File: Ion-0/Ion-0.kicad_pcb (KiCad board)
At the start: 4 copper layers, 99 parts, among them J1 Beaglebone-green-P9, J10 Conn_Heater, J11 Conn_01x02, J12 Conn_01x02, J13 Conn_01x04, J2 Beaglebone-green-P8, J3 Conn_02x06_Odd_Even, J4 Conn_02x06_Odd_Even, J5 Conn_02x06_Odd_Even, J6 Coaxial_Small, J7 Conn_01x02, J8 Conn_Heater, J9 Conn_Heater, Q1 IRLML6244, Q2 IRLML6244, Q3 IRLML6244, Q4 IRLML6244, U2 LMT84DCK, U3 BNO085, U4 TCA9617ADGKR, U5 LMT84DCK, U6 MAX-M10M-00B, U7 TPS3850H50DRCR, U8 SN65HVD230, U9 MS860702BA01-50, Y2 9HT10-32.768KBZF-T

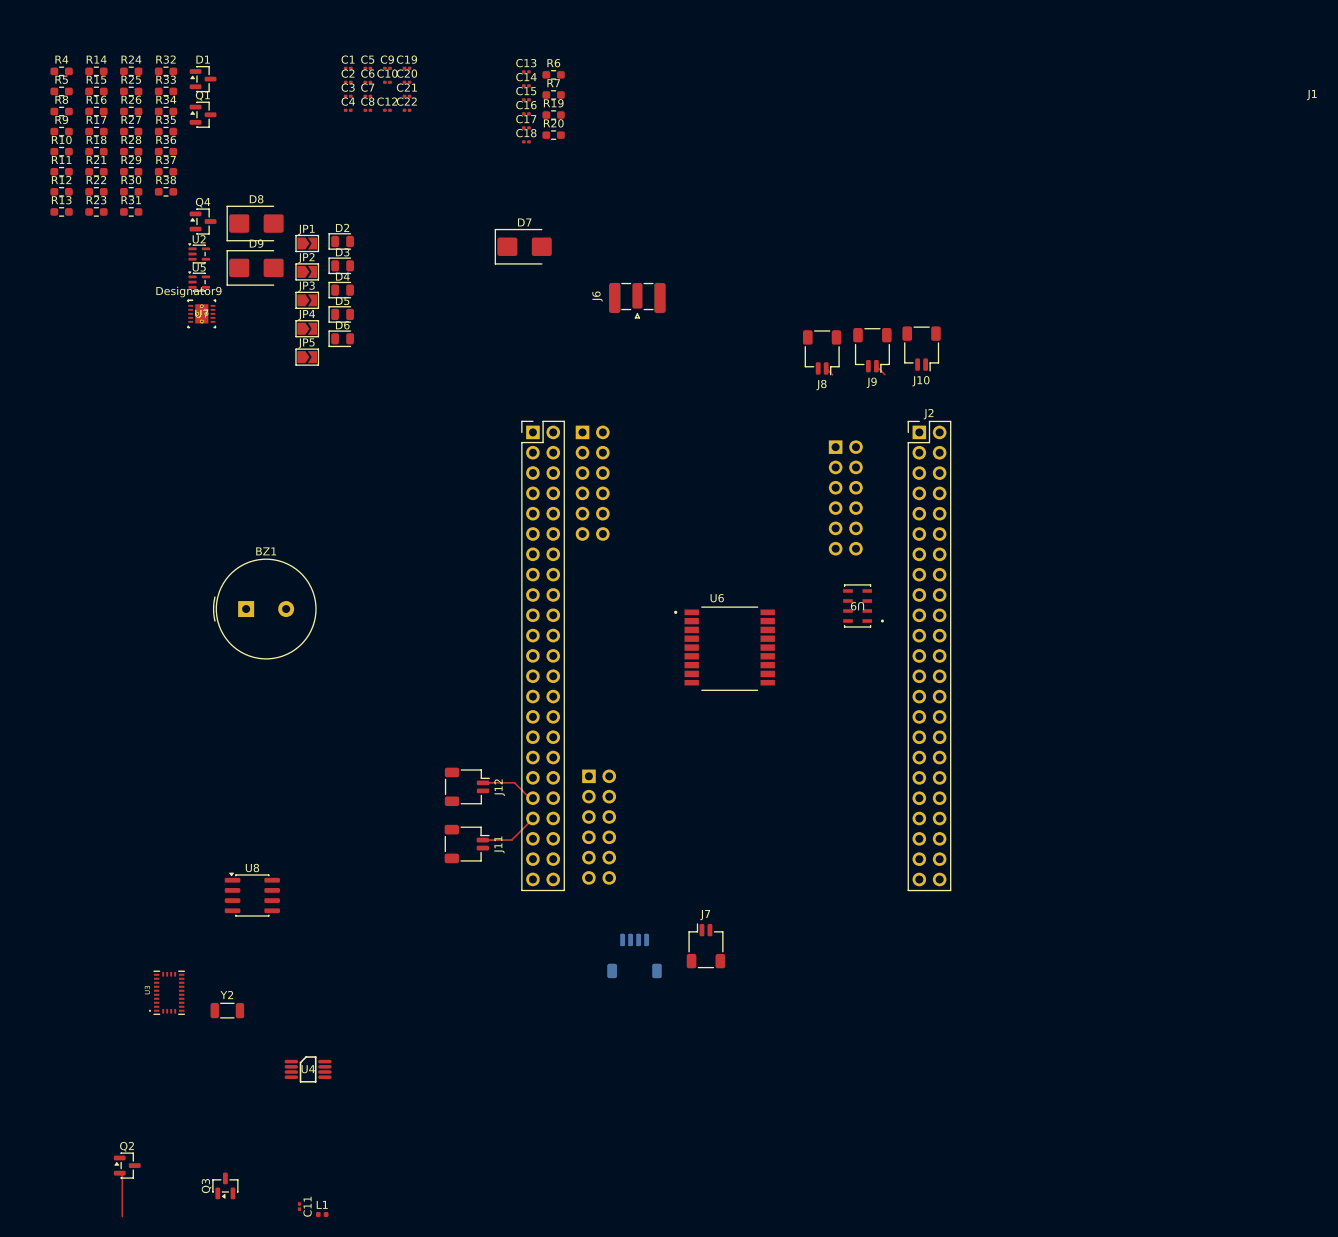
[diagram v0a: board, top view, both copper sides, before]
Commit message: midway through
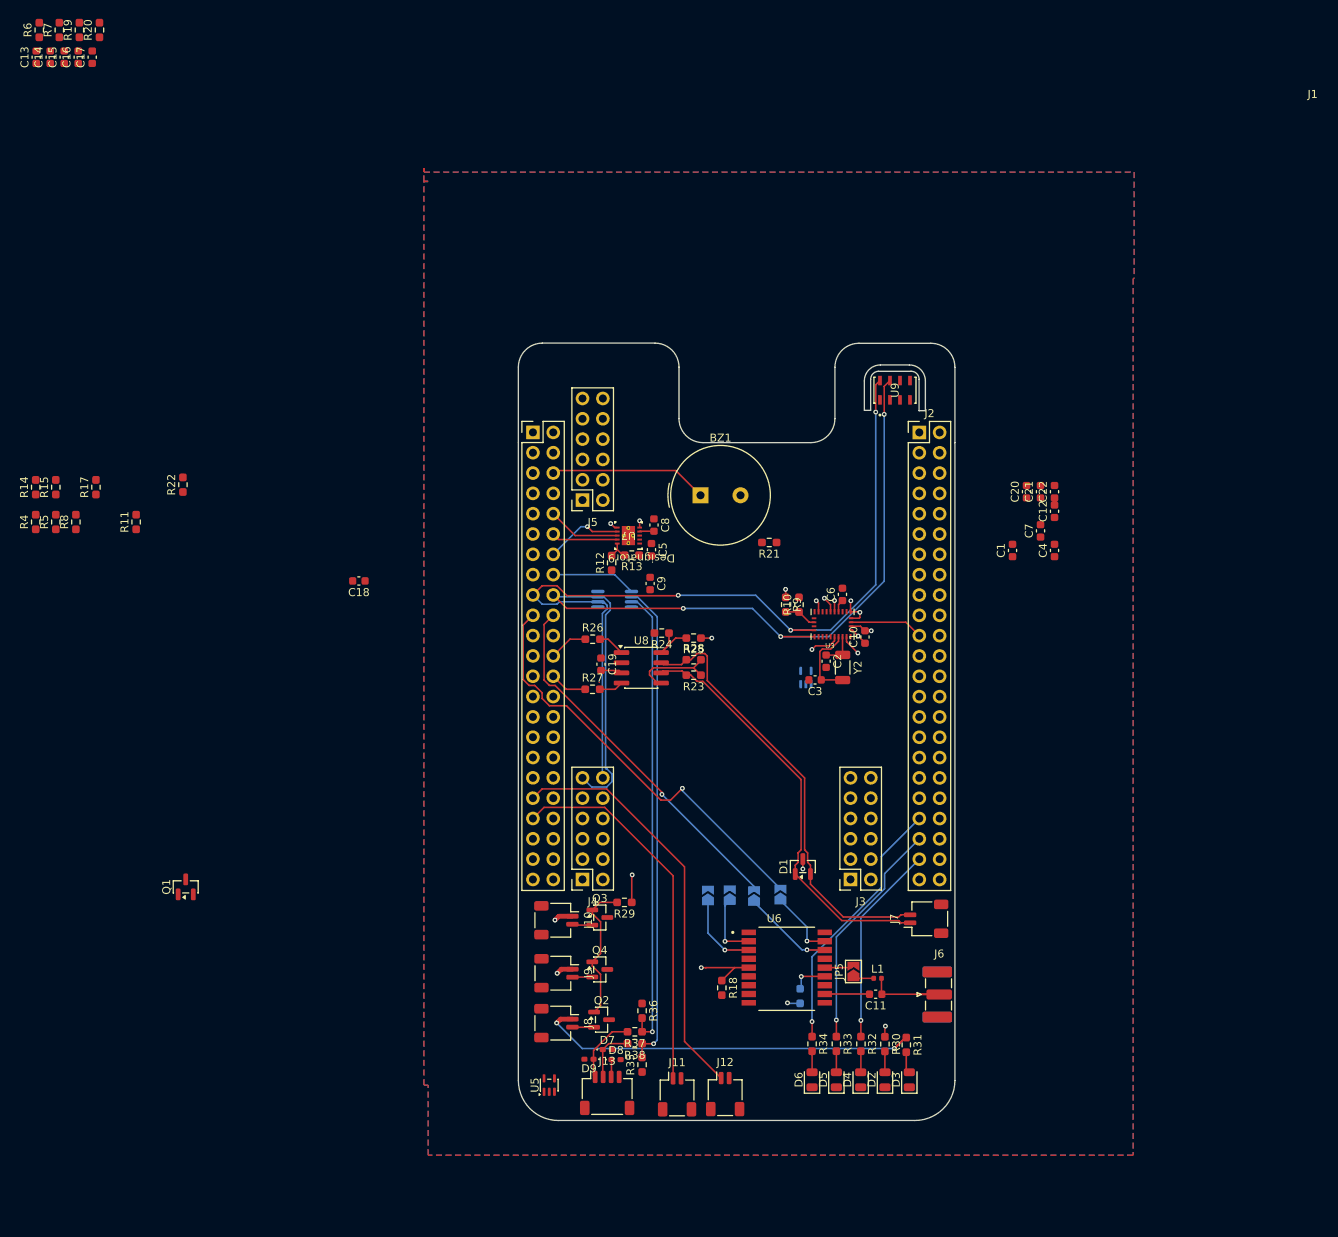
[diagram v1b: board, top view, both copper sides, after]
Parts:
- C1, C10, C11, C12, C13, C14, C15, C16, C17, C18, C19, C2, C20, C21, C22, C3, C4, C5, C6, C7, C8, C9: footprint Capacitor_SMD:C_0201_0603Metric -> Capacitor_SMD:C_0603_1608Metric
- D7, D8, D9: footprint Diode_SMD:D_SMB -> Diode_SMD:D_0402_1005Metric_Pad0.77x0.64mm_HandSolder
- J13, J3, J4, J5: moved to F.Cu
- JP1, JP2, JP3, JP4, R16, U2, U4: moved to B.Cu
- moved R32 149.4 mm to (129.3, 156.6), turned to -90 degrees
- moved R33 145.6 mm to (126.2, 156.6), turned to -90 degrees
- moved R31 142.2 mm to (135.0, 156.7), turned to -90 degrees
- moved R30 142.2 mm to (132.3, 156.6), turned to -90 degrees
- moved R34 141.8 mm to (123.2, 156.6), turned to -90 degrees
- moved R16 141.3 mm to (121.7, 150.6), turned to -90 degrees
- moved R35 130.9 mm to (101.9, 159.2), turned to 90 degrees
- moved R18 130.5 mm to (111.9, 149.6), turned to -90 degrees
- moved D2 124.8 mm to (132.3, 161.1), turned to 90 degrees
- moved D3 124.0 mm to (135.3, 161.1), turned to 90 degrees
- moved D1 123.7 mm to (122.0, 134.4), turned to 90 degrees
- moved R36 122.8 mm to (101.9, 152.5), turned to -90 degrees
- moved R37 122.4 mm to (101.0, 155.1), turned to 180 degrees
- moved R38 121.5 mm to (101.0, 156.6), turned to 180 degrees
- moved D4 118.1 mm to (129.3, 161.1), turned to 90 degrees
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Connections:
- D1 pad 1: /Sensor-bus-hat/CAN_P -> /Sensor-bus-hat/CAN_N
- D1 pad 2: /Sensor-bus-hat/CAN_N -> /Sensor-bus-hat/CAN_P
- J1 pad 12: unconnected-(J1-Pin_12-Pad12) -> /GPIO_60
- J1 pad 14: unconnected-(J1-Pin_14-Pad14) -> /GPIO_50
- J2 pad 3: /GPIO_38 -> unconnected-(J2-Pin_3-Pad3)
- J2 pad 5: /GPIO_34 -> unconnected-(J2-Pin_5-Pad5)
- J7 pad 1: /Sensor-bus-hat/CAN_P -> /Sensor-bus-hat/CAN_N
- J7 pad 2: /Sensor-bus-hat/CAN_N -> /Sensor-bus-hat/CAN_P
- R14 pad 2: /GPIO_38 -> /GPIO_60
- R33 pad 1: /GPIO_76 -> /GPIO_74
- R34 pad 1: /GPIO_74 -> /GPIO_76
- U7 pad 7: /GPIO_34 -> /GPIO_50
- U7 pad 9: /GPIO_38 -> /GPIO_60
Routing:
- net /I2C1_SDA: track 0.00 -> 111.0 mm, vias 0 -> 3
- net /I2C1_SCL: track 0.00 -> 108.8 mm, vias 0 -> 3
- net +5V: track 2.63 -> 92.0 mm, vias 0 -> 4
- net Net-(U4-SDAB): track 0.00 -> 61.0 mm, vias 0 -> 1
- net Net-(U4-SCLB): track 0.00 -> 58.5 mm, vias 0 -> 1
- net /Sensor-bus-hat/CAN_P: track 0.00 -> 54.7 mm
- net /I2C2_SCL: track 0.00 -> 53.3 mm, vias 0 -> 1
- net /Sensor-bus-hat/CAN_N: track 0.00 -> 52.2 mm
- net /I2C2_SDA: track 0.00 -> 46.1 mm, vias 0 -> 1
- net /AIN2: track 6.96 -> 51.8 mm
- net /AIN0: track 7.13 -> 47.0 mm
- net /GPIO_76: track 0.00 -> 32.9 mm, vias 0 -> 1
- net /GPIO_74: track 0.00 -> 29.0 mm, vias 0 -> 1
- net /GPIO_72: track 0.00 -> 25.2 mm, vias 0 -> 1
- net Net-(Q2-G): track 0.00 -> 17.9 mm
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- added copper zone on In2.Cu, net +3V3
- added copper zone on In2.Cu, net +5V
- added copper zone on B.Cu, net GND
- added copper zone on F.Cu, net GND
- added copper zone on In1.Cu, net GND
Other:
- board outline added: 54.6 x 97.2 mm
